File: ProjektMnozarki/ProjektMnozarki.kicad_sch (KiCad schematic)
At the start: 31 parts, among them IC1 SH8KC6TB1, U1 LM2903, U2 RC4580IDR, U3 RC4580IDR, U4 RC4580IDR, U5 TL431DBZ, U6 LMH6612MA, U7 LMH6612MA, U8 LT3045xDD

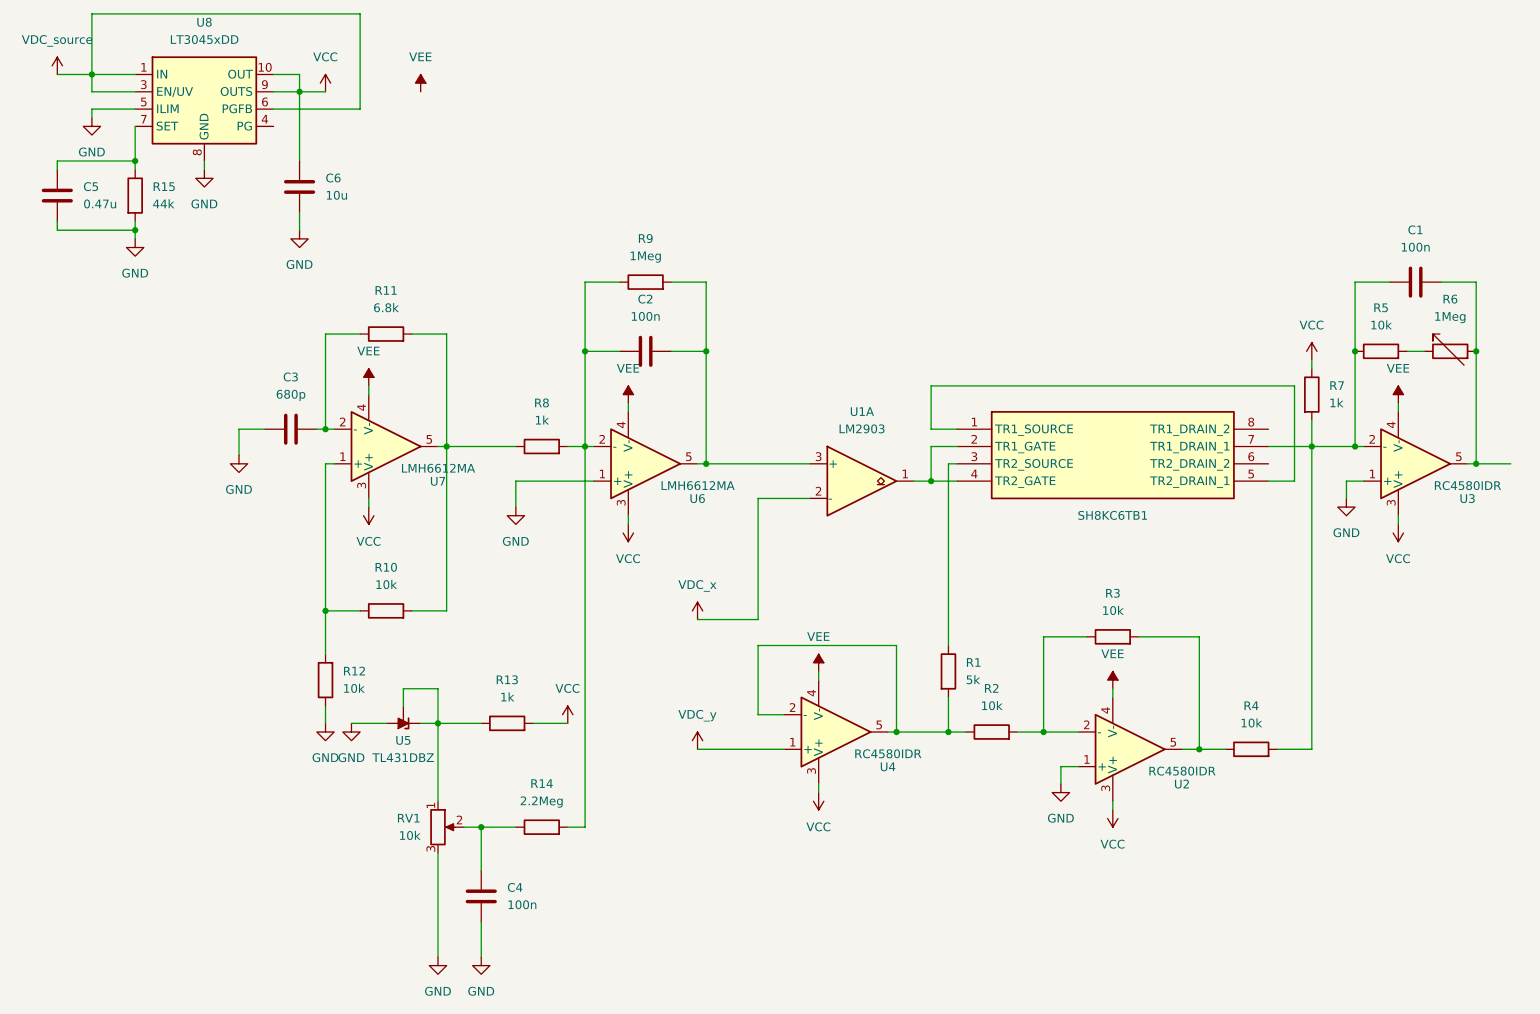
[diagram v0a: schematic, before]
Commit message: Add files via upload
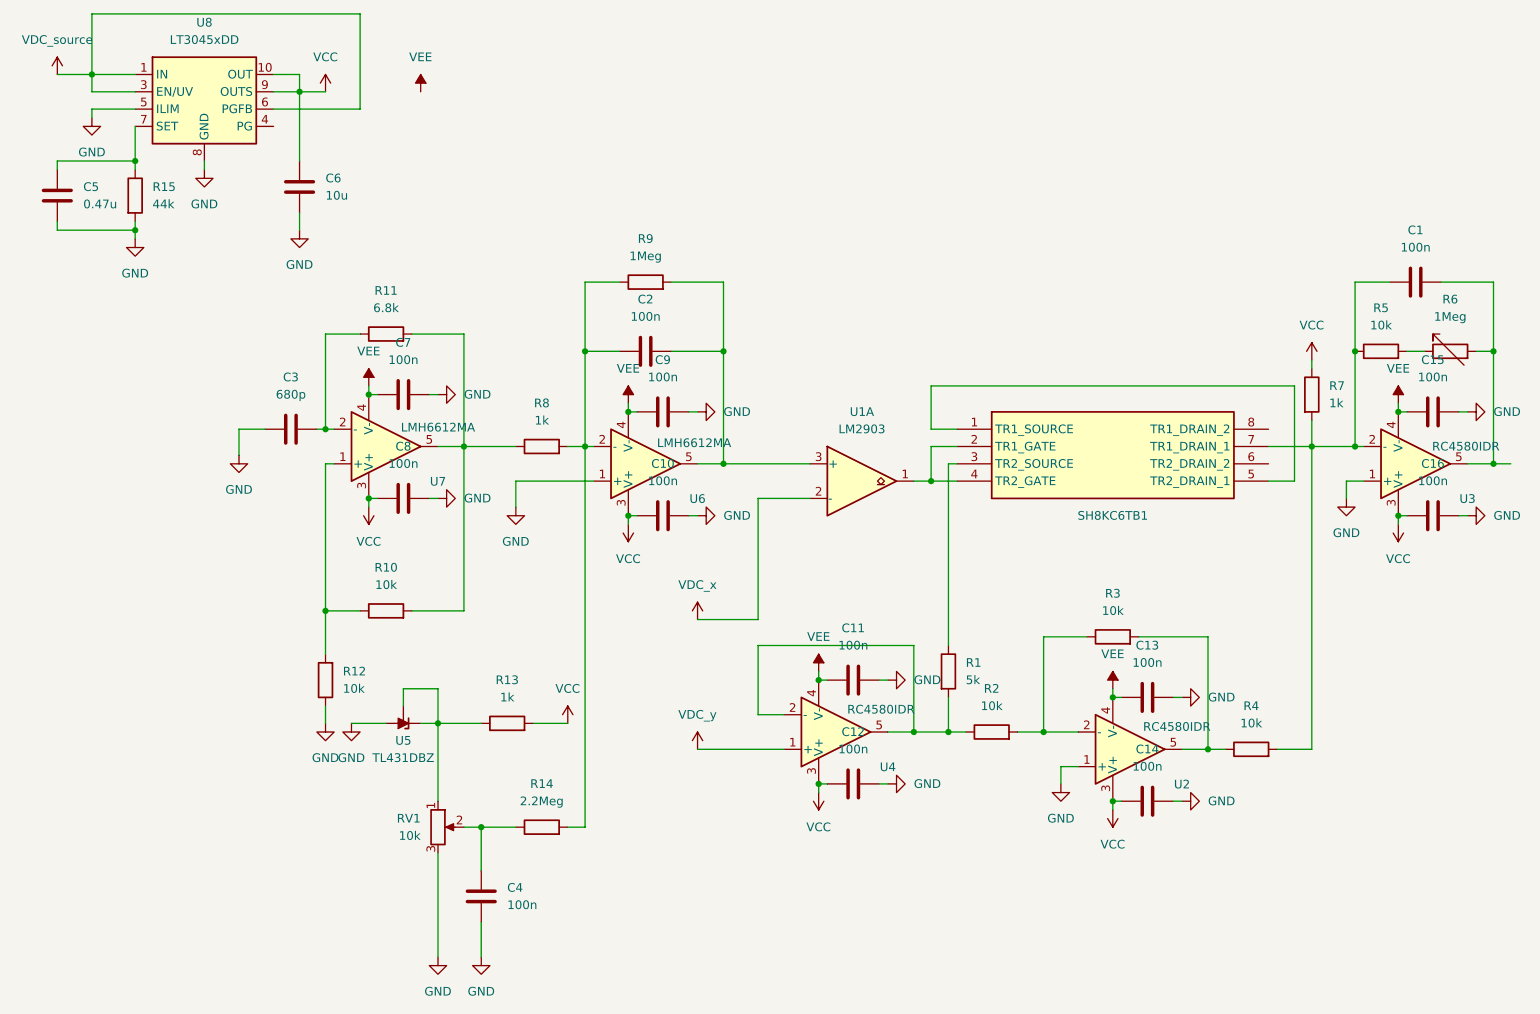
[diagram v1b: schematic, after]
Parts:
- added C10, C11, C12, C13, C14, C15, C16, C7, C8, C9: 100n, symbol Device:C
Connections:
- net GND: now also C10.2, C11.2, C12.2, C13.2, C14.2, C15.2, C16.2, C7.2, C8.2, C9.2
- net VCC: now also C10.1, C12.1, C14.1, C16.1, C8.1
- net VEE: now also C11.1, C13.1, C15.1, C7.1, C9.1
